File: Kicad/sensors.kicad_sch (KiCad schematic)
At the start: 13 parts, among them J5 Conn_02x03_Top_Bottom, J6 Conn_02x03_Top_Bottom, J7 Conn_02x03_Top_Bottom, J8 Conn_02x03_Top_Bottom, U1 ITR8307, U2 ITR8307, U3 ITR8307

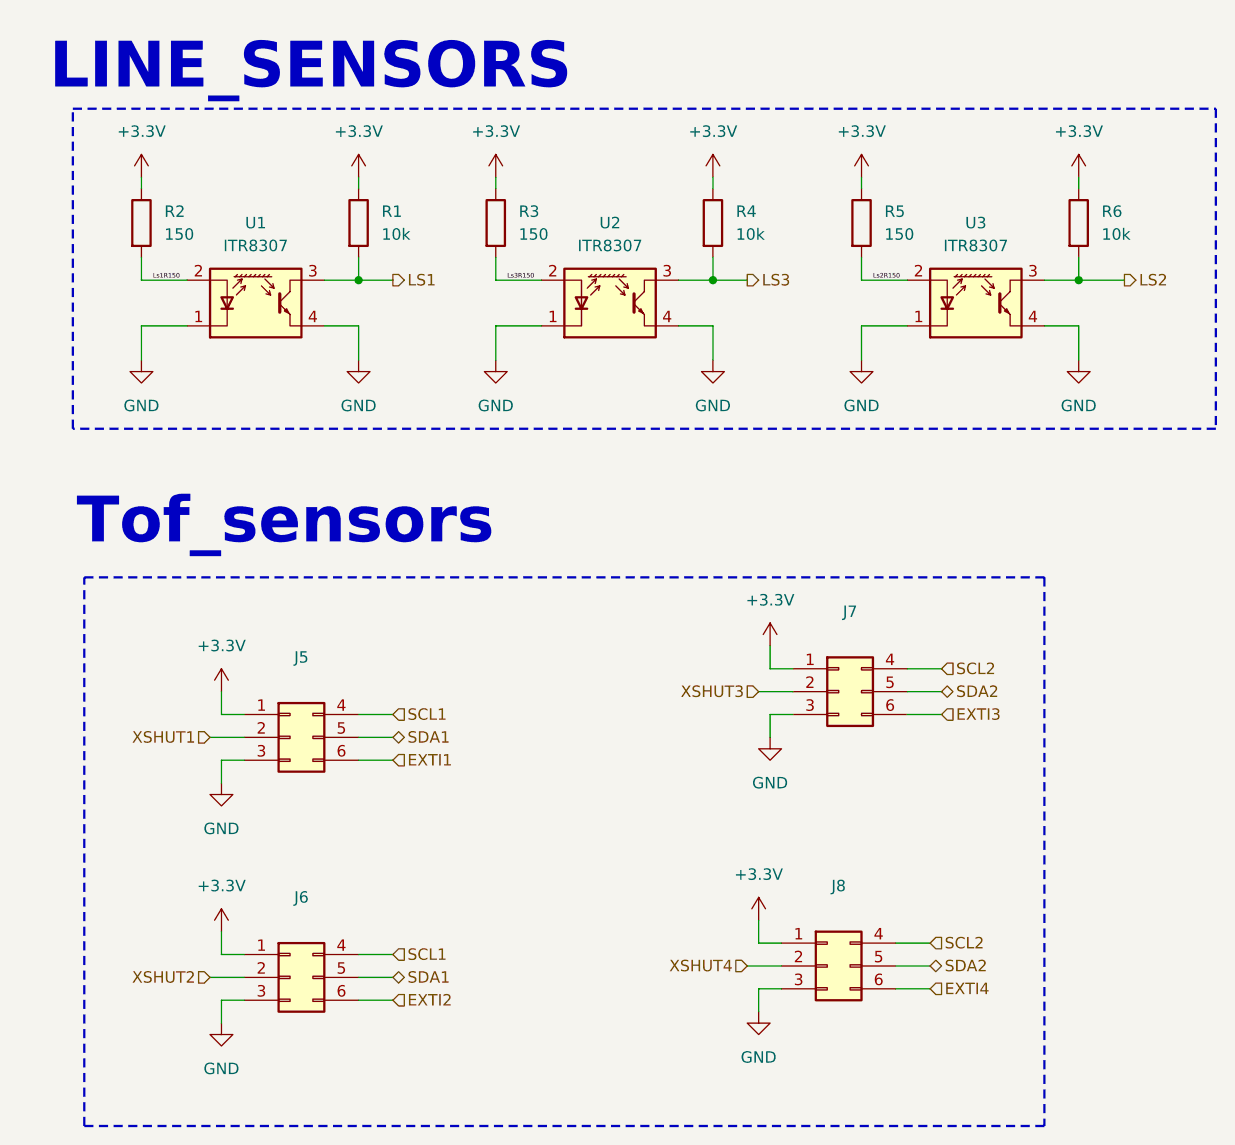
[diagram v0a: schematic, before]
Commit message: not small changes
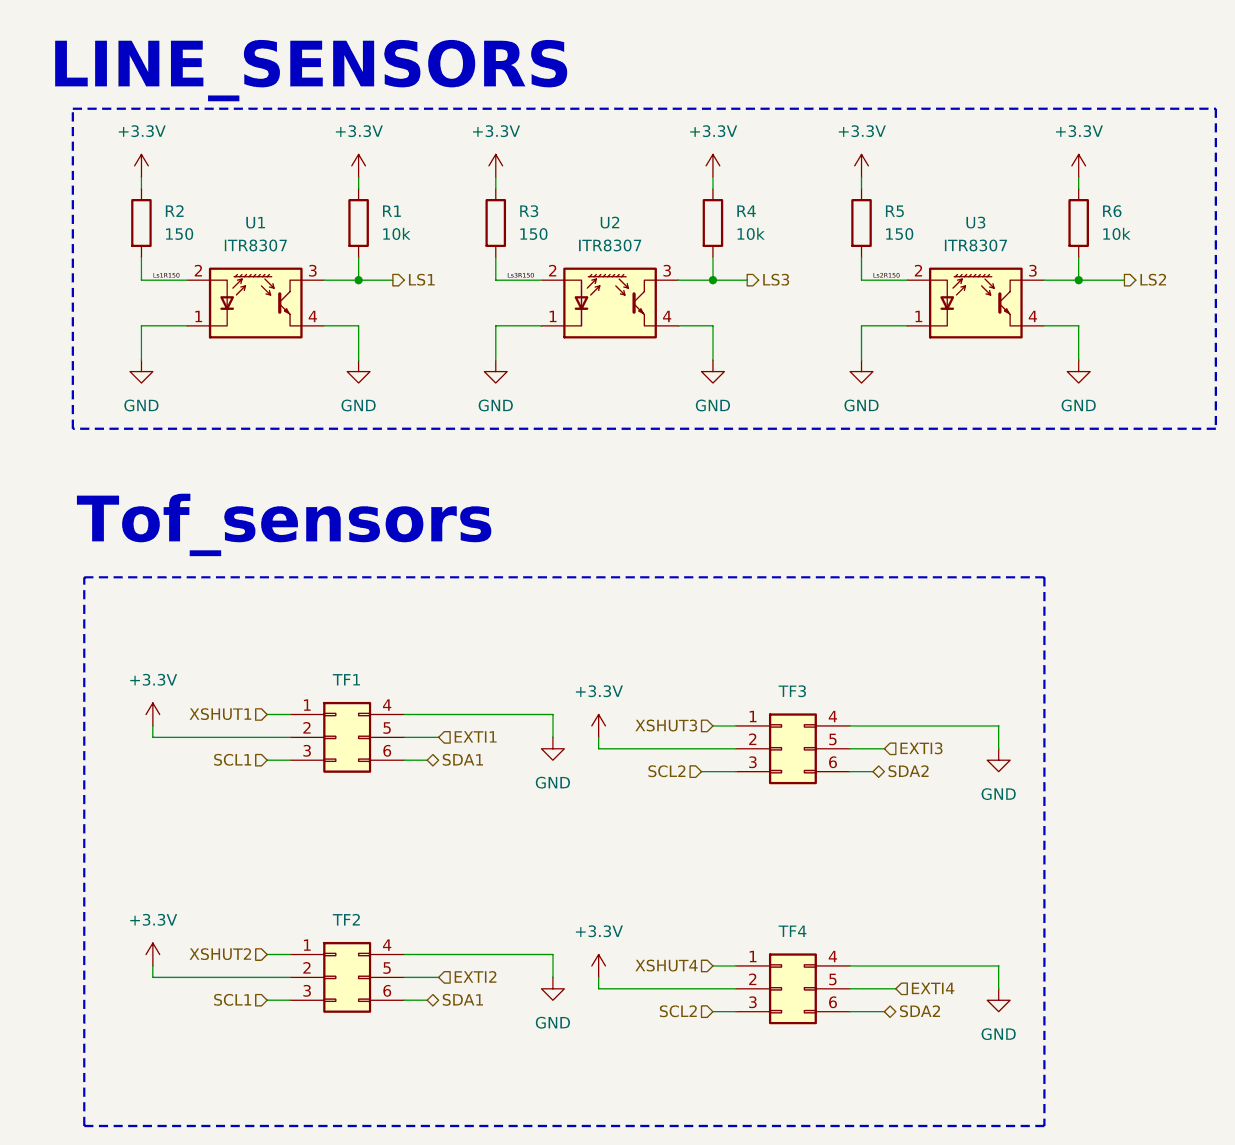
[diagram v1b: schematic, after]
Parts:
- removed J6, J7, J8: Conn_02x03_Top_Bottom, Connector_PinSocket_2.54mm:PinSocket_2x03_P2.54mm_Vertical, symbol Connector_Generic:Conn_02x03_Top_Bottom
- added TF2, TF3, TF4: Conn_02x03_Top_Bottom, Connector_PinHeader_2.54mm:PinHeader_2x03_P2.54mm_Vertical, symbol Connector_Generic:Conn_02x03_Top_Bottom
- TF1: renamed from J5; footprint Connector_PinSocket_2.54mm:PinSocket_2x03_P2.54mm_Vertical -> Connector_PinHeader_2.54mm:PinHeader_2x03_P2.54mm_Vertical
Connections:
- net +3.3V: now also TF1.2 (Pin_2), TF2.2 (Pin_2), TF3.2 (Pin_2), TF4.2 (Pin_2); no longer TF1.1 (Pin_1)
- net EXTI1: now also TF1.5 (Pin_5); no longer TF1.6 (Pin_6)
- net EXTI2: now also TF2.5 (Pin_5)
- net EXTI3: now also TF3.5 (Pin_5)
- net EXTI4: now also TF4.5 (Pin_5)
- net GND: now also TF1.4 (Pin_4), TF2.4 (Pin_4), TF3.4 (Pin_4), TF4.4 (Pin_4); no longer TF1.3 (Pin_3)
- net SCL1: now also TF1.3 (Pin_3), TF2.3 (Pin_3); no longer TF1.4 (Pin_4)
- net SCL2: now also TF3.3 (Pin_3), TF4.3 (Pin_3)
- net SDA1: now also TF1.6 (Pin_6), TF2.6 (Pin_6); no longer TF1.5 (Pin_5)
- net SDA2: now also TF3.6 (Pin_6), TF4.6 (Pin_6)
- net XSHUT1: now also TF1.1 (Pin_1); no longer TF1.2 (Pin_2)
- net XSHUT2: now also TF2.1 (Pin_1)
- net XSHUT3: now also TF3.1 (Pin_1)
- net XSHUT4: now also TF4.1 (Pin_1)
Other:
- moved on the sheet: TF1
